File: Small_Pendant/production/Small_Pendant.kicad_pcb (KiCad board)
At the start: 4 copper layers, 180.6 x 75.6 mm, 4 parts

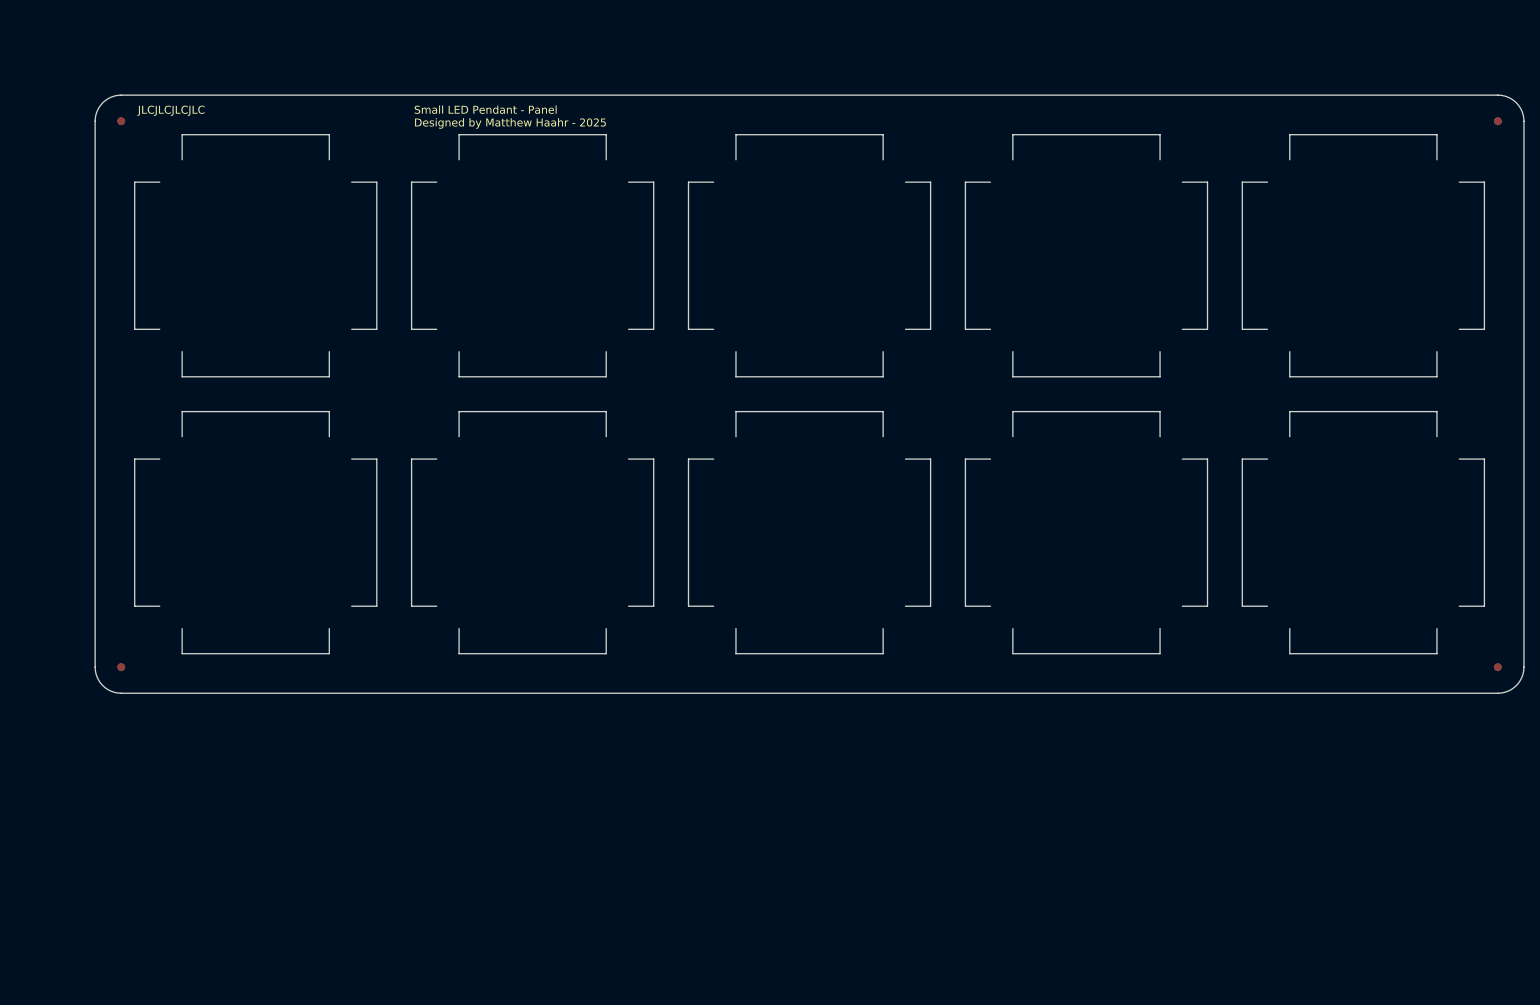
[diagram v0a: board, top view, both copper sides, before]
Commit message: [HW] Improve panelization frame
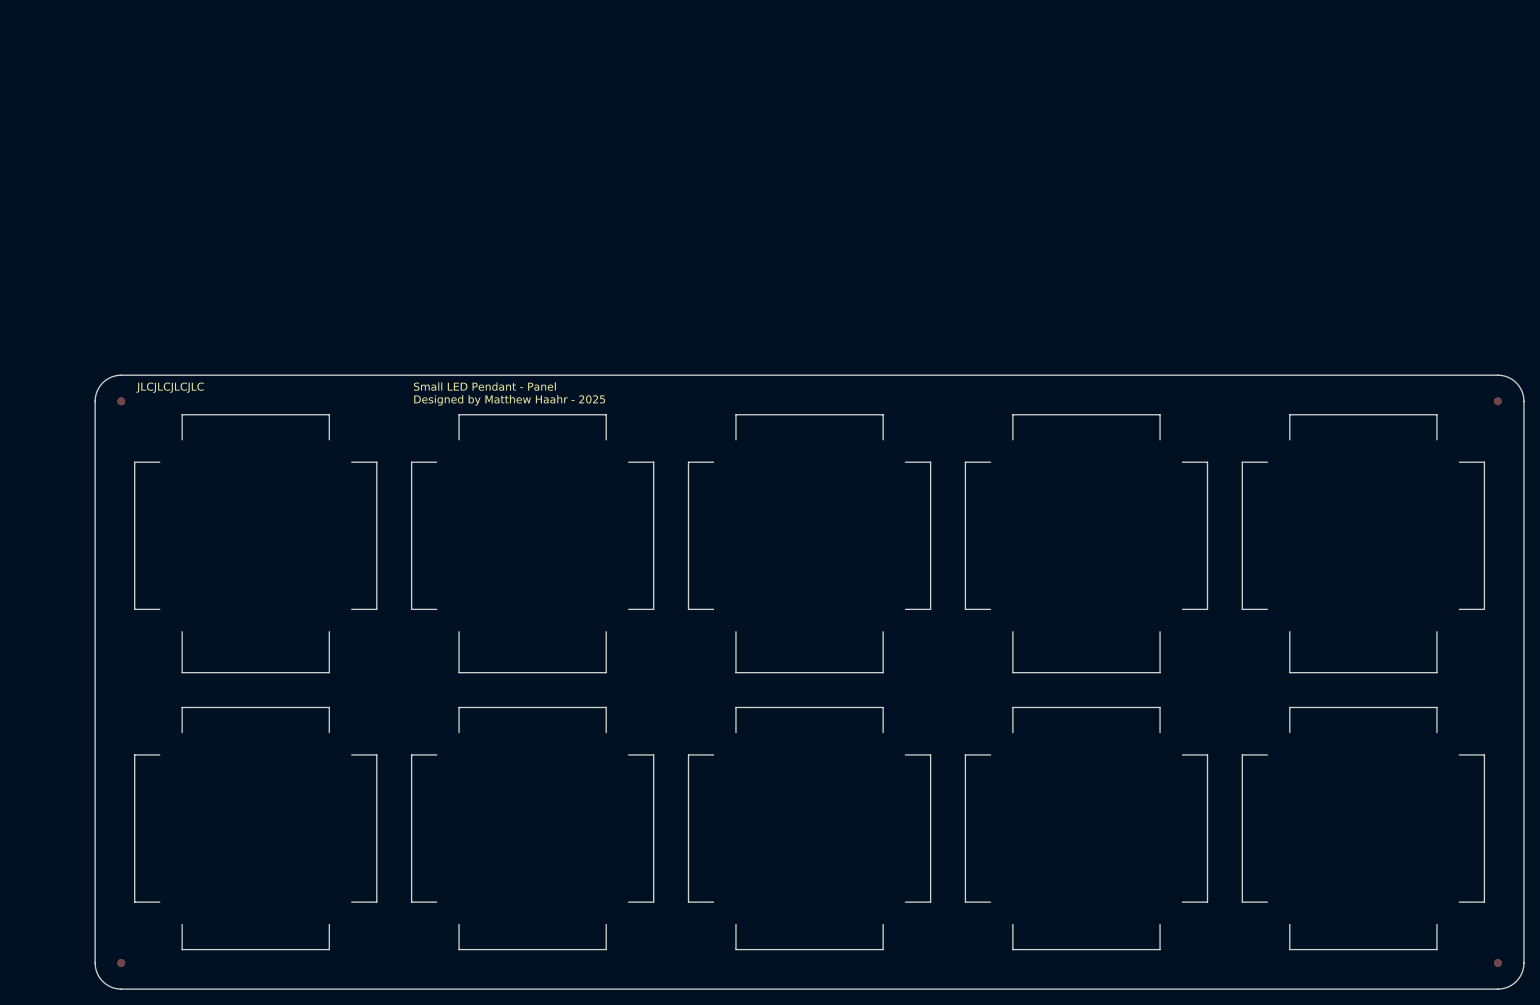
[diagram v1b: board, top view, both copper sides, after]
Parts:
- moved REF** 204.0 mm to (207.0, 139.4), turned to 180 degrees
- moved REF** 204.0 mm to (33.0, 139.4), turned to 180 degrees
- moved REF** 177.2 mm to (33.0, 68.4), turned to 180 degrees
- moved REF** 177.2 mm to (207.0, 68.4), turned to 180 degrees
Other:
- board size 180.6 x 75.6 mm -> 180.6 x 77.6 mm
- board text added: "LED Boards"
- board text added: "MCU Boards USB Down"

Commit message: [HW] Add Fillets to panels
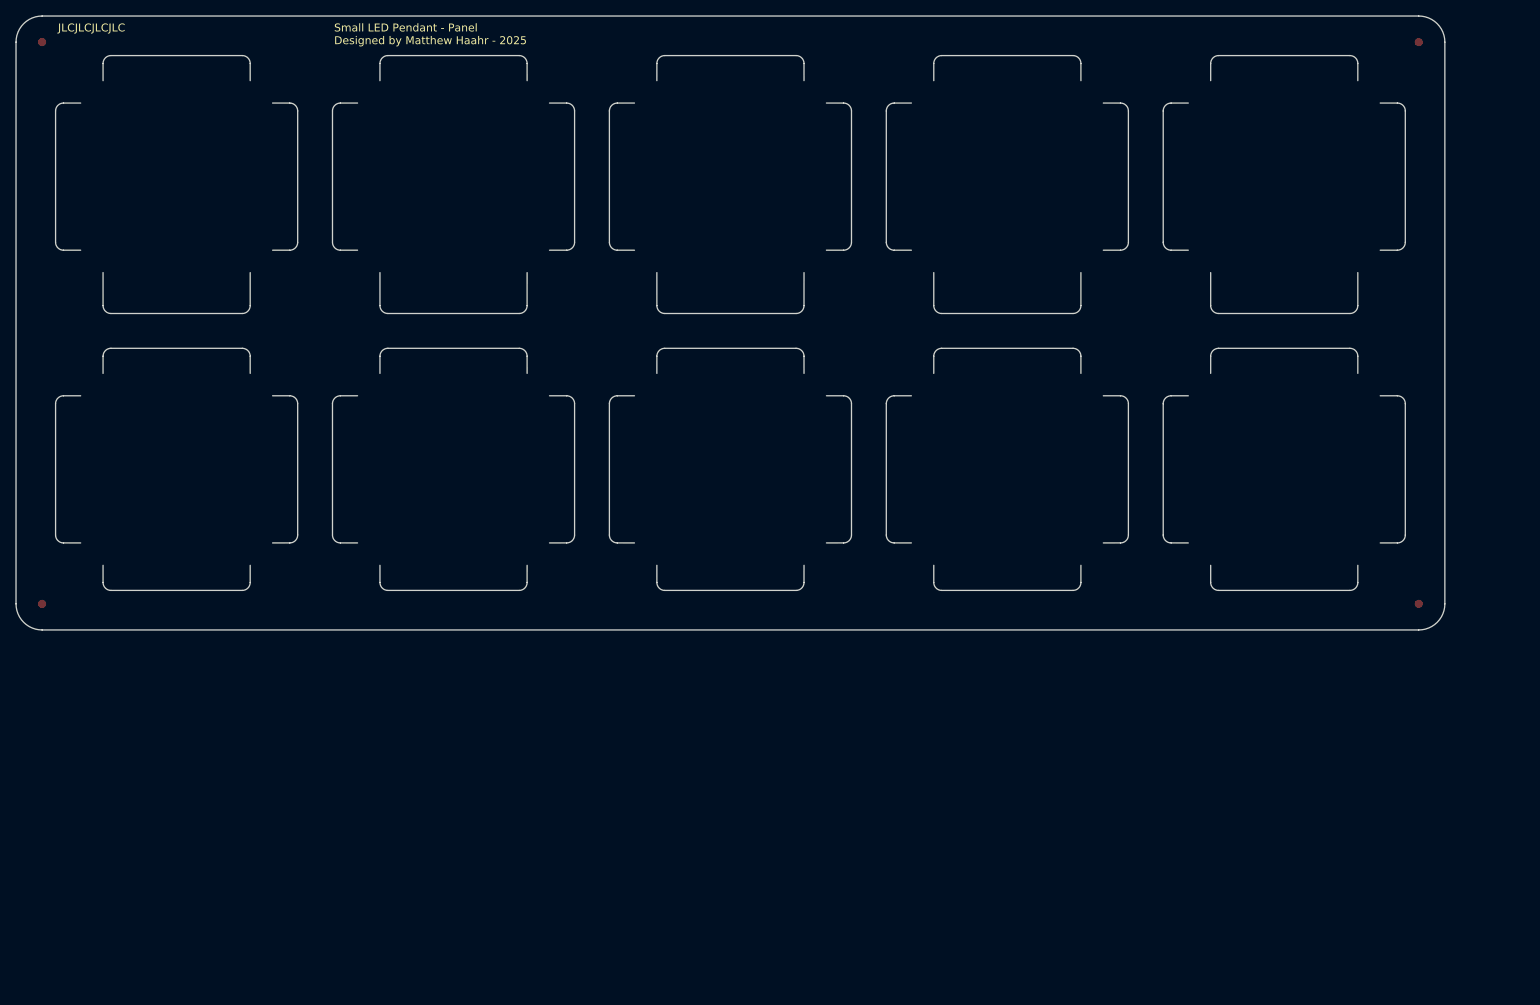
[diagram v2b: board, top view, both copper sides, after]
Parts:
- moved REF** 46.5 mm to (23.0, 23.0)
- moved REF** 46.5 mm to (23.0, 94.0)
- moved REF** 46.5 mm to (197.0, 94.0)
- moved REF** 46.5 mm to (197.0, 23.0)
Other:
- outline, holes or cut-outs redrawn
